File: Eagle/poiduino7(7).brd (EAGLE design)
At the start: 69.6 x 56.9 mm, 20 parts, among them K1 TS-1109, Y1 16MHZ

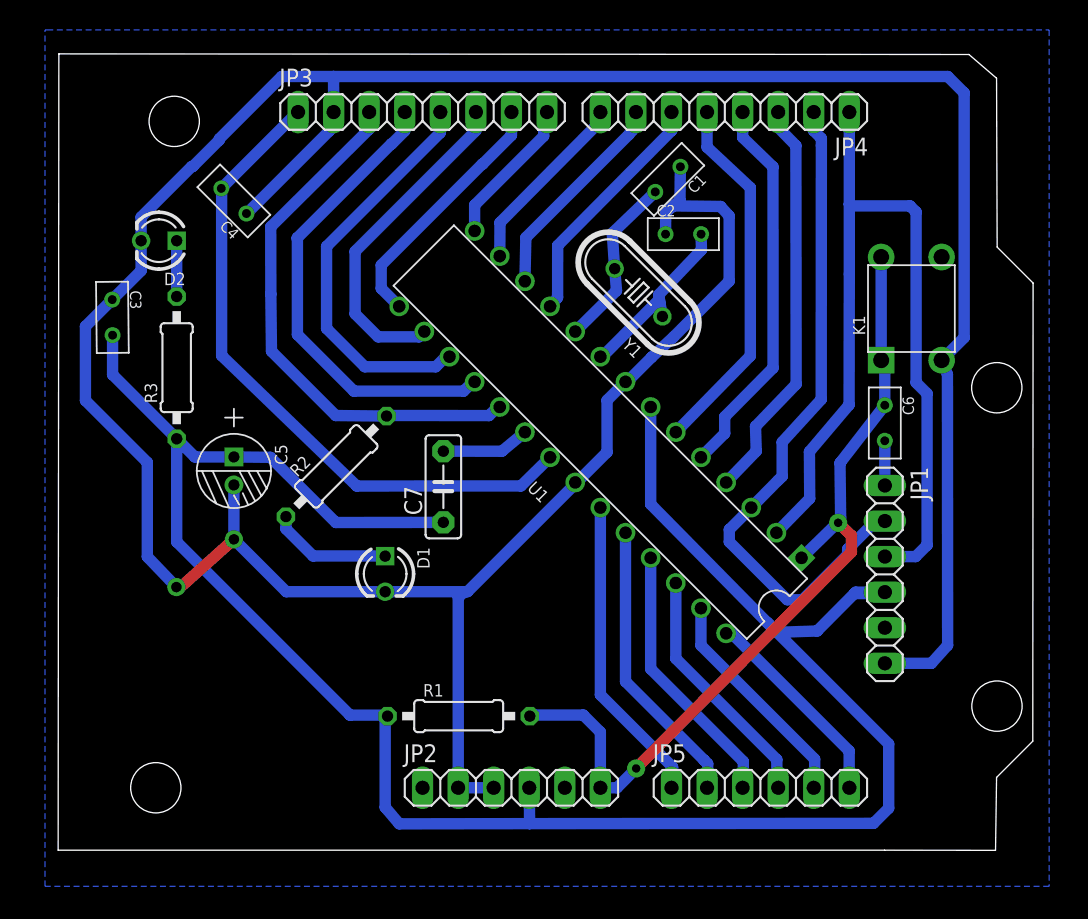
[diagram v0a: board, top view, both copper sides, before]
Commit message: fix pads board
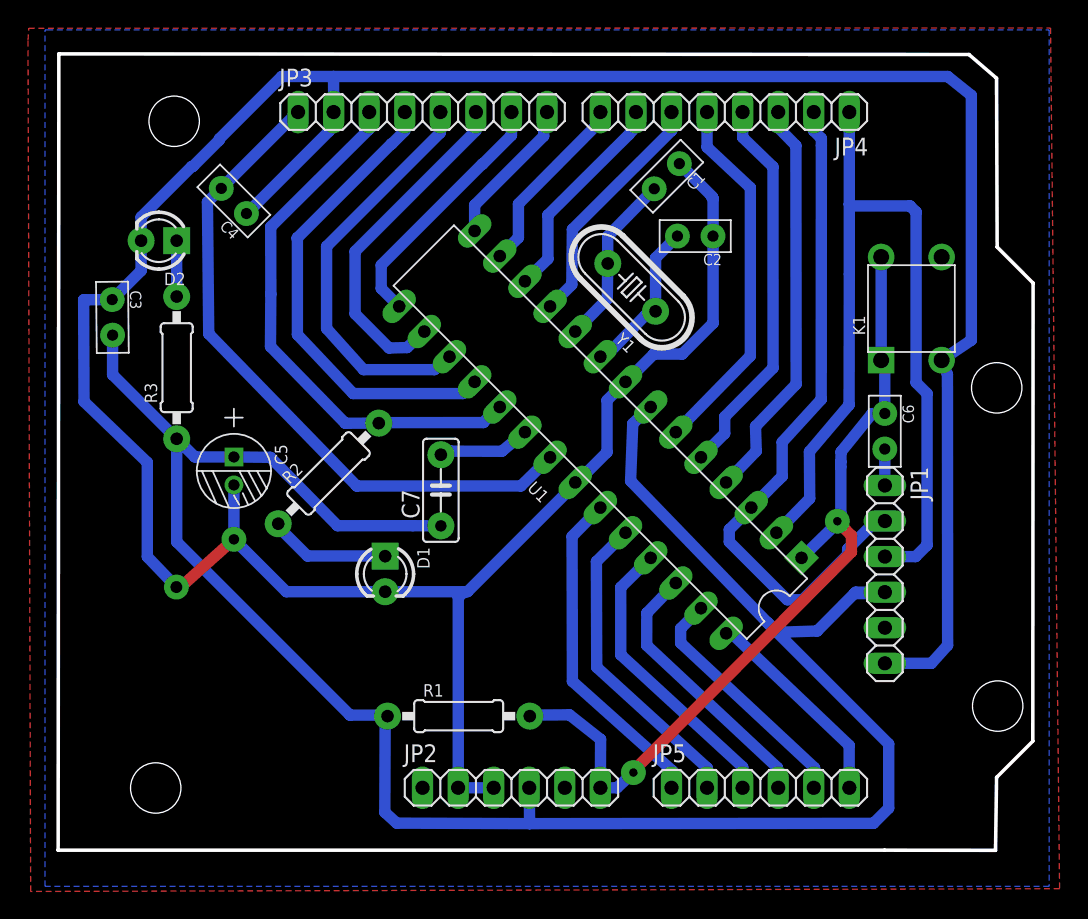
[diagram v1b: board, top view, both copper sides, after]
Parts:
- C1, C2: value 18pf -> 10nf
- C3, C4, C6: value 0.1uf -> 10nf
- C5: value 1uf -> 100uf
- JP1: value (none) -> jp1
- JP2: value (none) -> jp2
- JP3: value (none) -> jp3
- JP4: value (none) -> jp4
- JP5: value (none) -> jp5
- U1: value (none) -> Atmega328p
- moved C2 0.86 mm to (45.5, 43.9), turned to 180 degrees
- moved R2 0.75 mm to (19.2, 26.9)
- moved Y1 0.62 mm to (40.9, 40.2)
- moved C6 0.59 mm to (59.0, 30.0)
- moved C7 0.31 mm to (27.3, 25.7)
- moved C1 0.23 mm to (43.5, 48.2)
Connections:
- removed net CTS: JP1.5
- removed net N$34: JP2.1
- removed net N$38: JP2.5
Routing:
- net GND: track 241.4 -> 238.7 mm
- net XTAL1: track 14.3 -> 12.2 mm
- net A2: track 19.2 -> 21.2 mm
- net A1: track 20.7 -> 22.6 mm
- net A3: track 17.7 -> 19.6 mm
- net A0: track 22.2 -> 24.1 mm
- net A4-SDA: track 16.2 -> 17.6 mm
- net VCC: track 153.8 -> 155.0 mm
- net PIN10: track 23.8 -> 24.4 mm
- net AREF: track 47.8 -> 48.4 mm
- net DTR: track 3.19 -> 2.60 mm
- added copper zone on layer 1, net GND
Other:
- outline, holes or cut-outs redrawn
